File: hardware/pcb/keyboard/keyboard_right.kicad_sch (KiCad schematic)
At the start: 35 parts, among them J1 SM04B-SRSS-TB, J2 PJ320D, J3 HRO_TYPE-C-31-M-12, J4 HRS_FH34SRJ-06S-0.5SH(50), SW29 PTS845, U3 PRTR5V0U2X, U4 XC6220B331MR-G, U5 STM32G431KBTx, U6 24FC01T-I/OT, Y1 8MHz 10pF

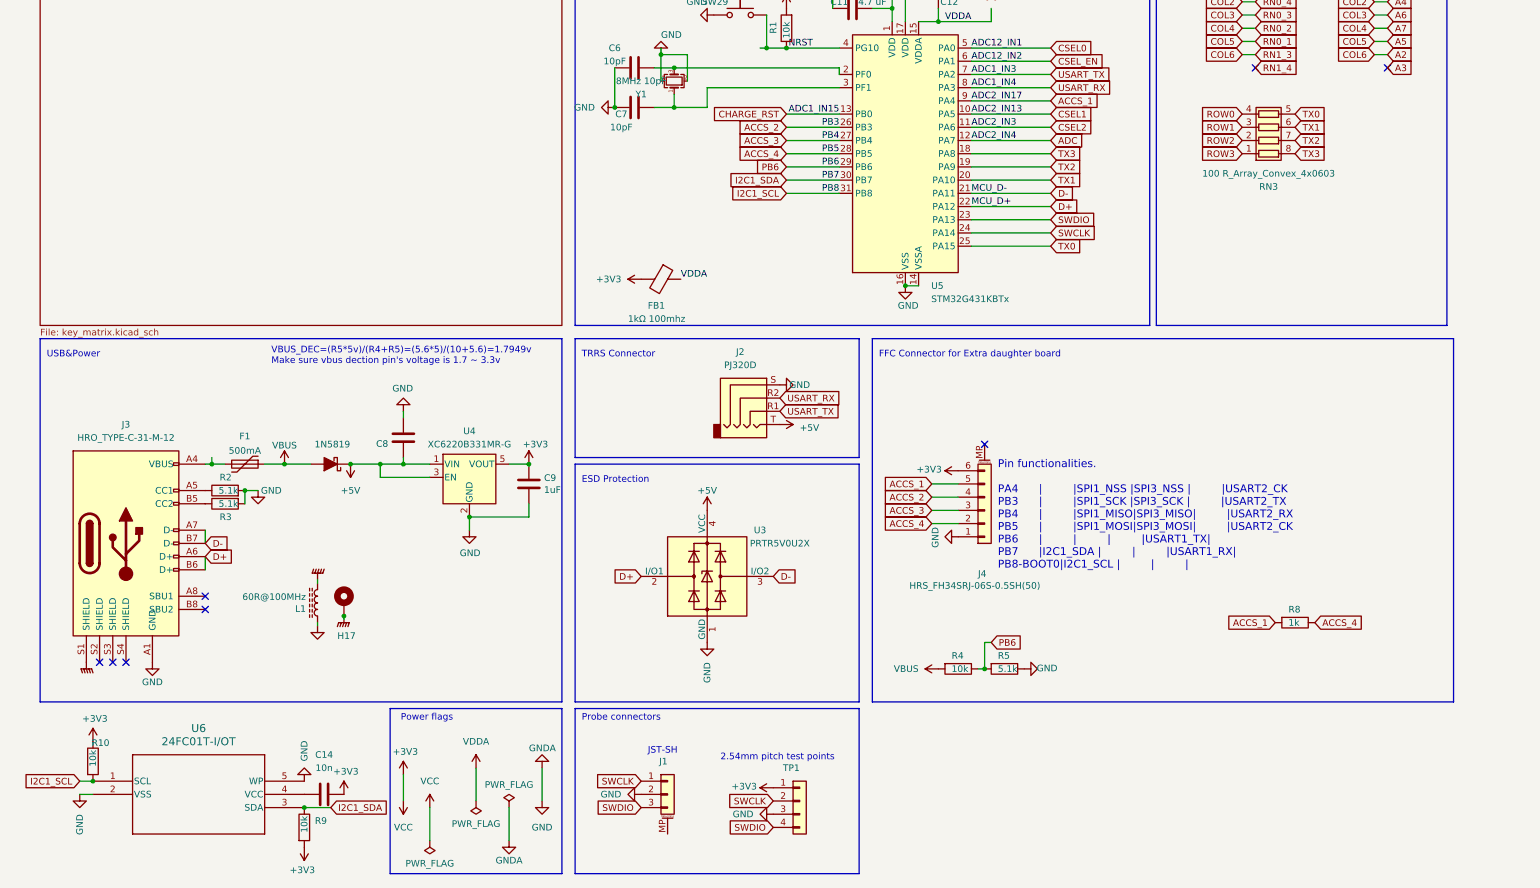
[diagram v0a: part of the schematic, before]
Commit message: update schema.
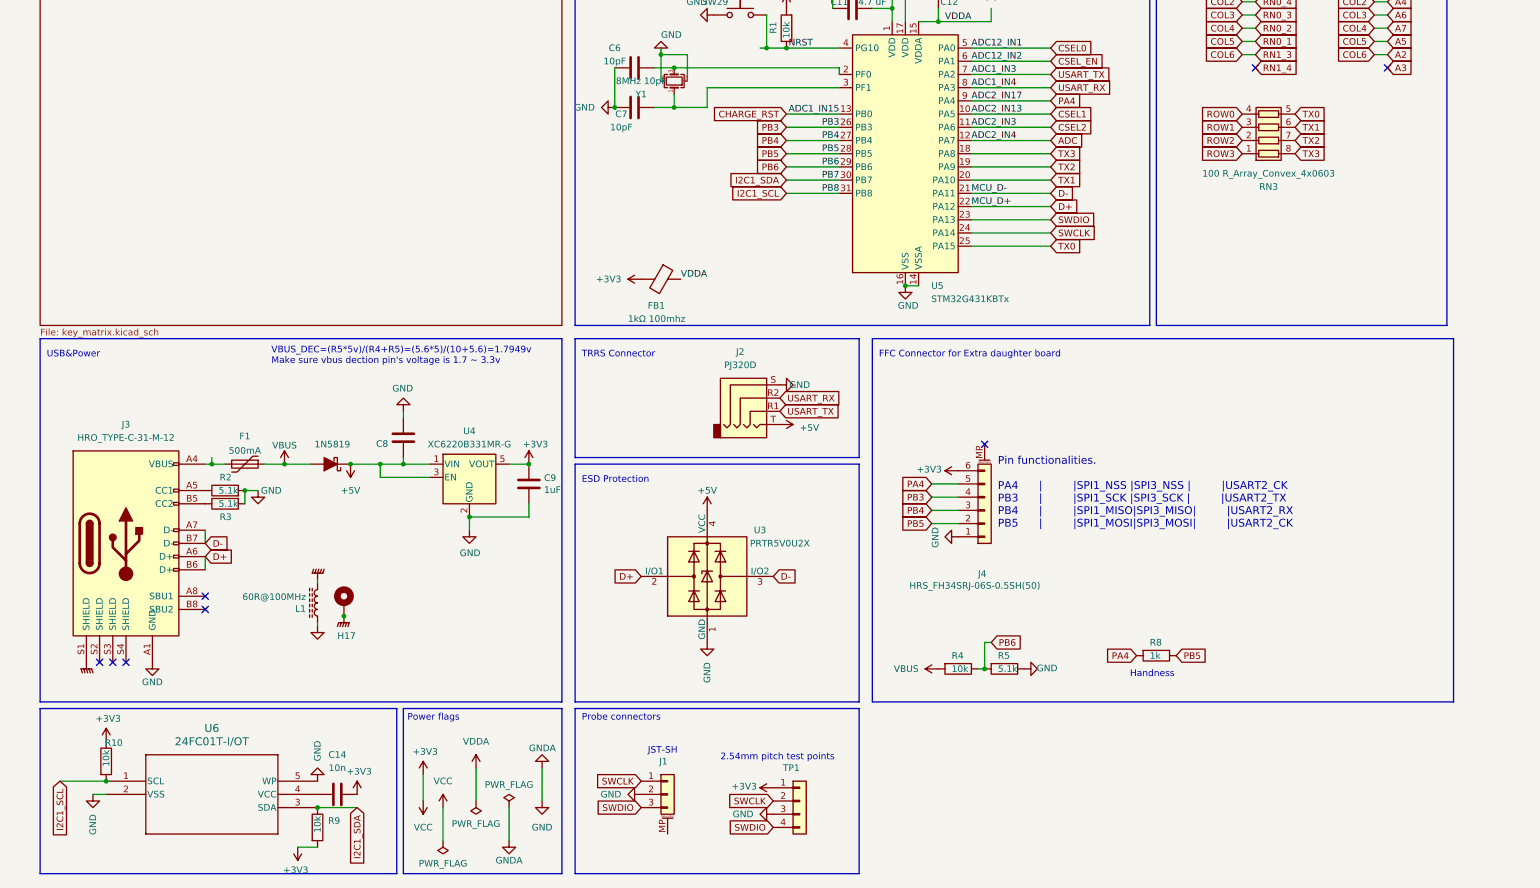
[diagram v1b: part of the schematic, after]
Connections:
- net ACCS_1 renamed PA4
- net ACCS_2 renamed PB3
- net ACCS_3 renamed PB4
- net ACCS_4 renamed PB5
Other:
- note added: "Handness"
- note added: "Pin functionalities. PA4 | |SPI1_NSS |SPI3_NSS | |USART2_CK PB3 | |SPI1_SCK |SPI3_SCK | |USART2_TX PB4 | |SPI1_MISO|SPI3_MISO| |USART2_RX PB5 | |SPI1_MOSI|SPI3_MOSI| |USART2_CK"
- note removed: "Pin functionalities. PA4 | |SPI1_NSS |SPI3_NSS | |USART2_CK PB3 | |SPI1_SCK |SPI3_SCK | |USART2_TX PB4 | |SPI1_MISO|SPI3_MISO| |USART2_RX PB5 | |SPI1_MOSI|SPI3_MOSI| |USART2_CK PB6 | | | |USART1_TX| PB7 |I2C1_SDA | | |USART1_RX| PB8-BOOT0|I2C1_SCL | | |"
- company: (none) -> https://github.com/daehyeok/Corne_EEC
- moved on the sheet: C14, R10, R8, R9, U6
